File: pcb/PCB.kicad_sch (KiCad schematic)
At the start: 35 parts, among them J1 Conn_01x15, J2 USB_C_Receptacle_USB2.0, J3 Conn_01x15, J4 TC2030, J5 Conn_01x04, SW1 SW_Push, SW2 SW_Push, U1 SN65HVD230, U2 AMS1117-3.3, U3 STM32F103C8T6, Y1 8MHz

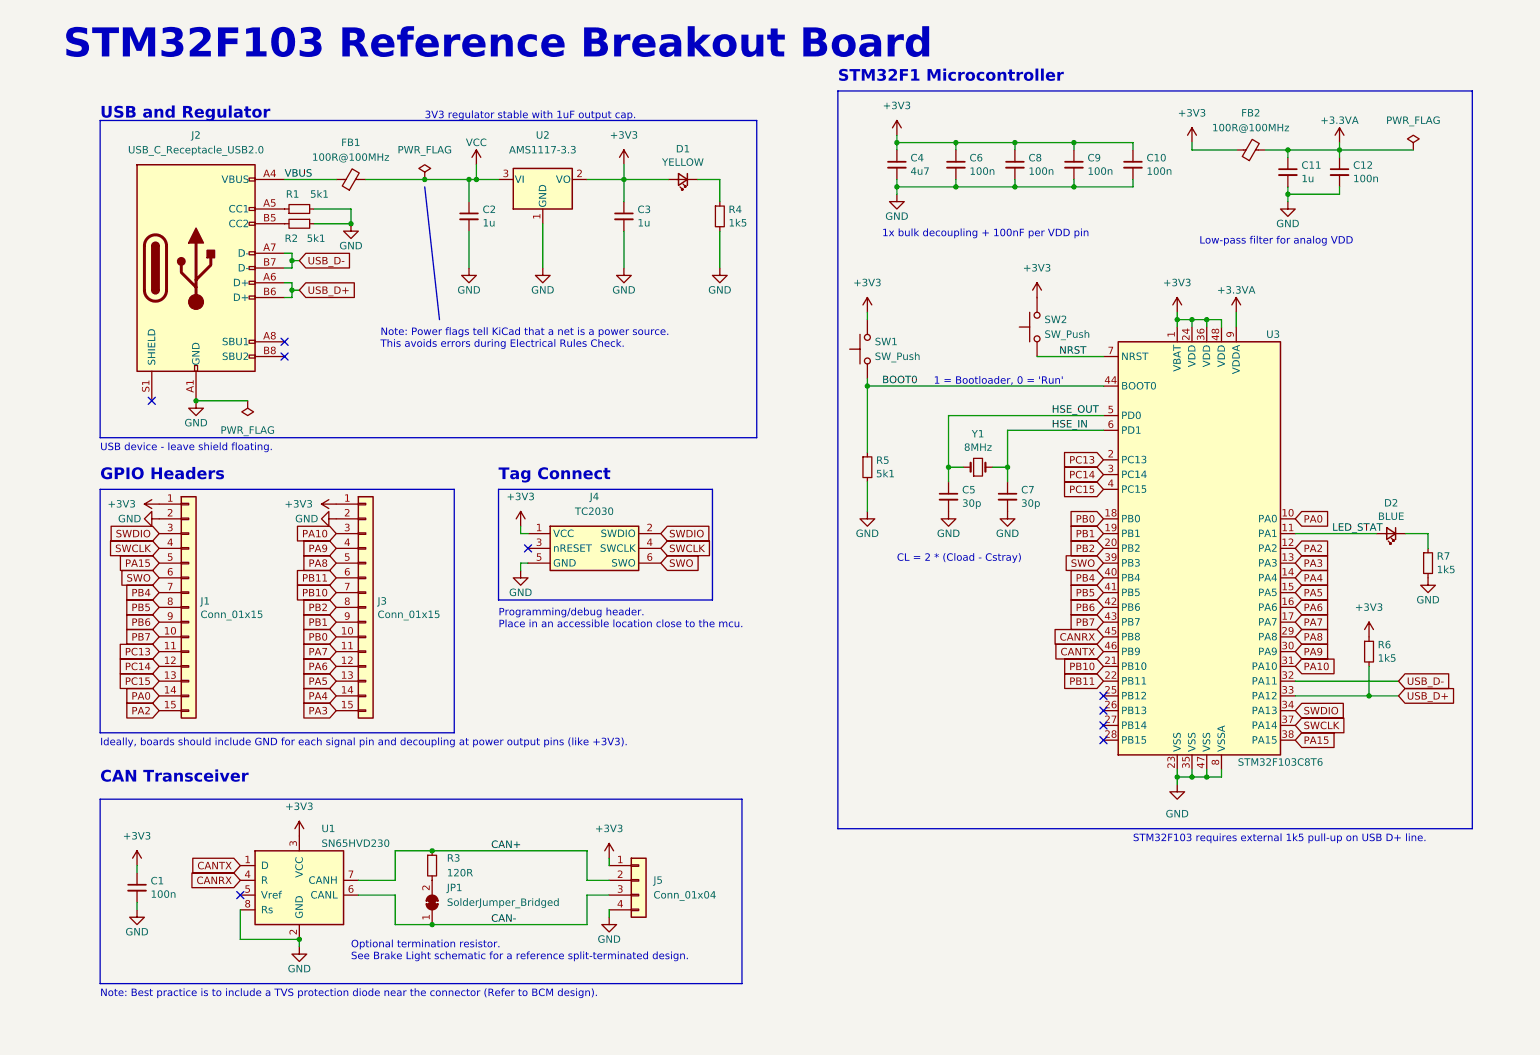
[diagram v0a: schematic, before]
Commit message: Finished schematic
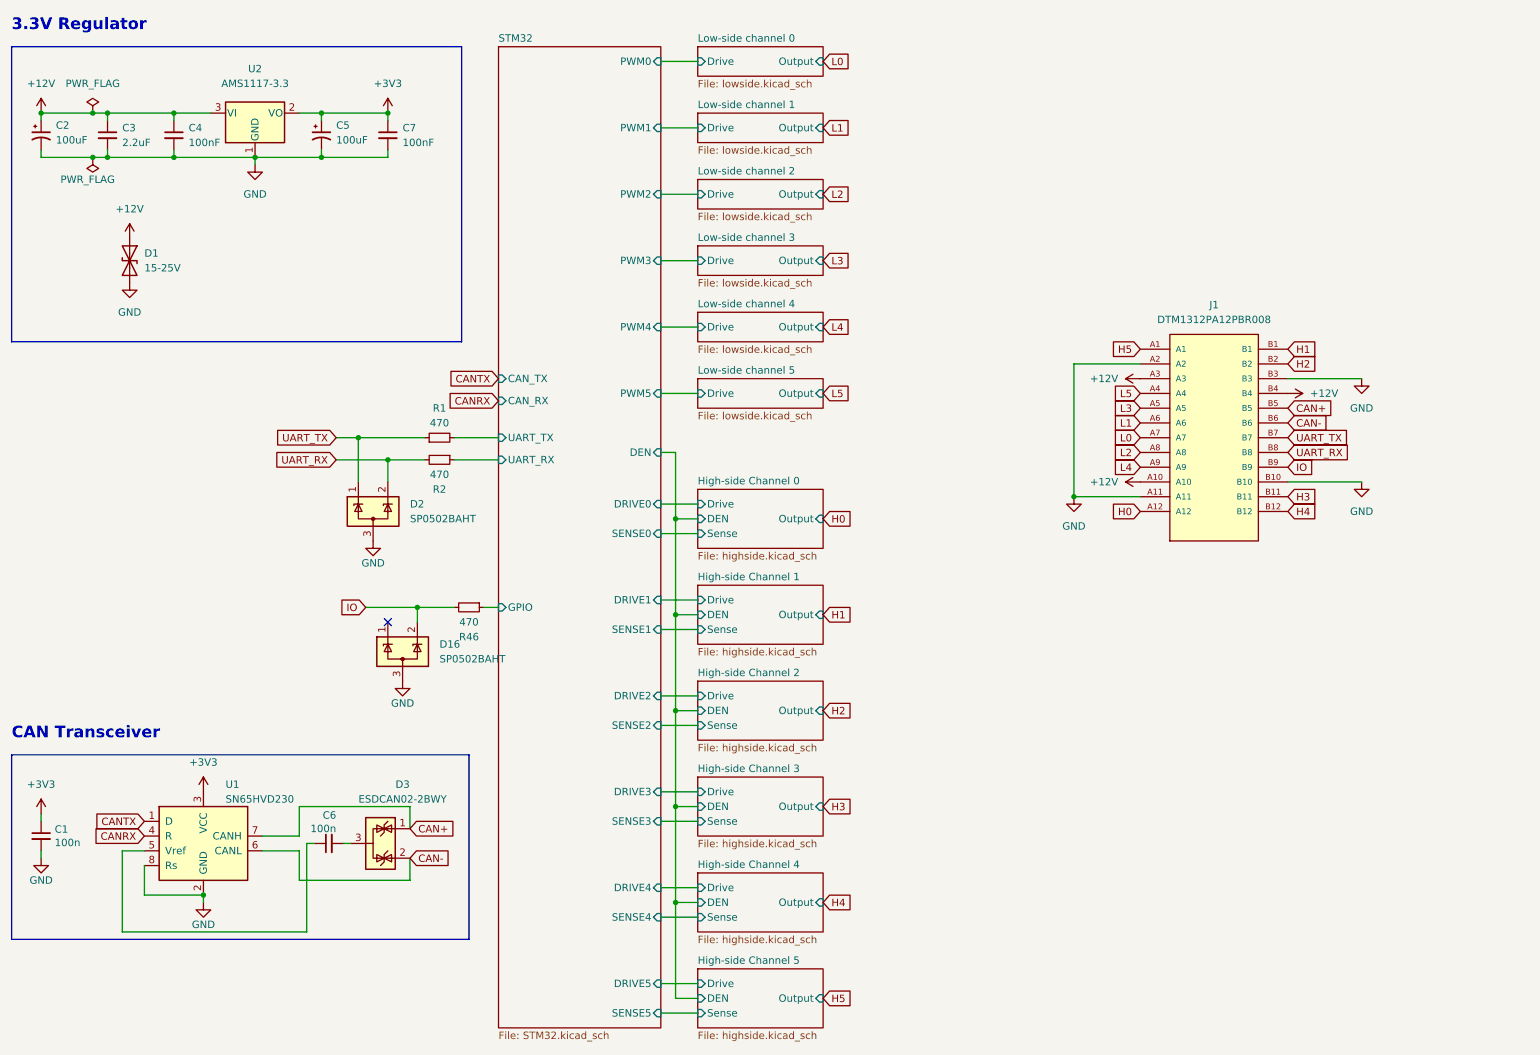
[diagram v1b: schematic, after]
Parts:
- removed C10, C12, C8, C9: 100n, Capacitor_SMD:C_0402_1005Metric, symbol Device:C_Small
- removed C11, C2: 1u, Capacitor_SMD:C_0603_1608Metric, symbol Device:C_Small
- removed C5: 30p, Capacitor_SMD:C_0402_1005Metric, symbol Device:C_Small
- removed D1: YELLOW, LED_SMD:LED_0603_1608Metric, symbol Device:LED_Small
- removed D2: BLUE, LED_SMD:LED_0603_1608Metric, symbol Device:LED_Small
- removed FB1, FB2: 100R@100MHz, Resistor_SMD:R_0805_2012Metric, symbol Device:FerriteBead_Small
- removed J1, J3: Conn_01x15, Connector_PinHeader_2.54mm:PinHeader_1x15_P2.54mm_Vertical, symbol Connector_Generic:Conn_01x15
- removed J2: USB_C_Receptacle_USB2.0, Connector_USB:USB_C_Receptacle_HRO_TYPE-C-31-M-12, symbol Connector:USB_C_Receptacle_USB2.0
- removed J4: TC2030, Connector:Tag-Connect_TC2030-IDC-NL_2x03_P1.27mm_Vertical, symbol TC2030:TC2030
- removed J5: Conn_01x04, Connector_PinHeader_2.54mm:PinHeader_1x04_P2.54mm_Vertical, symbol Connector_Generic:Conn_01x04
- removed JP1: SolderJumper_Bridged, Jumper:SolderJumper-2_P1.3mm_Bridged_RoundedPad1.0x1.5mm, symbol Jumper:SolderJumper_2_Bridged
- removed R3: 120R, Resistor_SMD:R_0402_1005Metric, symbol Device:R_Small
- removed R4, R6, R7: 1k5, Resistor_SMD:R_0402_1005Metric, symbol Device:R_Small
- removed R5: 5k1, Resistor_SMD:R_0402_1005Metric, symbol Device:R_Small
- removed SW1, SW2: SW_Push, Button_Switch_SMD:SW_Push_1P1T_NO_CK_KSC7xxJ, symbol Switch:SW_Push
- removed U3: STM32F103C8T6, Package_QFP:LQFP-48_7x7mm_P0.5mm, symbol MCU_ST_STM32F1:STM32F103C8Tx
- removed Y1: 8MHz, Crystal:Crystal_SMD_5032-2Pin_5.0x3.2mm, symbol Device:Crystal_Small
- added C2, C5: 100uF, Capacitor_SMD:CP_Elec_6.3x7.7, symbol Device:C_Polarized_Small_US
- added D1: 15-25V, Diode_SMD:D_SMA, symbol Device:D_TVS
- added D16, D2: SP0502BAHT, Package_TO_SOT_SMD:SOT-23, symbol Power_Protection:SP0502BAHT
- added D3: ESDCAN02-2BWY, Package_TO_SOT_SMD:SOT-23, symbol Power_Protection:NUP2105L
- added J1: DTM1312PA12PBR008, DTM13-12PA-12PB:TE_DTM1312PA12PBR008, symbol DTM1312PA12PBR008:DTM1312PA12PBR008
- added R46: 470, Resistor_SMD:R_0603_1608Metric, symbol Device:R_Small
- C3: value 1u -> 2.2uF; footprint Capacitor_SMD:C_0603_1608Metric -> Capacitor_SMD:C_0805_2012Metric; LCSC C15849 -> (none)
- C4: value 4u7 -> 100nF; LCSC C19666 -> (none)
- C7: value 30p -> 100nF; footprint Capacitor_SMD:C_0402_1005Metric -> Capacitor_SMD:C_0603_1608Metric; LCSC C1570 -> (none)
- R1, R2: value 5k1 -> 470; footprint Resistor_SMD:R_0402_1005Metric -> Resistor_SMD:R_0603_1608Metric; LCSC C25905 -> (none)
- U2: LCSC C6186 -> (none)
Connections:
- net HSE_IN is gone; now on net +3V3: C7.1
- net +3V3: now also C5.1; no longer C3.1, C4.1, C6.1
- net CAN+: now also D3.1 (K), J1.B5
- net CAN-: now also D3.2 (K), J1.B6
- net GND: now also C2.2, C5.2, D1.2 (A2), D16.3 (A), D2.3 (A), J1.A11, J1.A2, J1.B10, J1.B3; no longer C6.2, R1.2, R2.1
- net UART_TX: now reaches R1.1
- net UART_TX: now also D2.1 (K), J1.B7
- net UART_RX: now reaches R2.2
- net UART_RX: now also D2.2 (K), J1.B8
- net at U1.5 (Vref): now also C6.1
- net VCC renamed +12V
- net +12V: now also C3.1, C4.1, C2.1, D1.1 (A1), J1.A10, J1.A3, J1.B4
- new net: C6.2, D3.3 (A)
- new net H0: J1.A12
- new net H1: J1.B1
- new net H2: J1.B2
- new net H3: J1.B11
- new net H4: J1.B12
- new net H5: J1.A1
- new net IO: D16.2 (K), J1.B9, R46.2
- new net L0: J1.A7
- new net L1: J1.A6
- new net L2: J1.A8
- new net L3: J1.A5
- new net L4: J1.A9
- new net L5: J1.A4
- new net STM32/GPIO: R46.1
- new net STM32/UART_RX: R2.1
- new net STM32/UART_TX: R1.2
- no-connect marks 9 -> 1
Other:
- added sheet High-side Channel 0 (highside.kicad_sch)
- added sheet High-side Channel 1 (highside.kicad_sch)
- added sheet High-side Channel 2 (highside.kicad_sch)
- added sheet High-side Channel 3 (highside.kicad_sch)
- added sheet High-side Channel 4 (highside.kicad_sch)
- added sheet High-side Channel 5 (highside.kicad_sch)
- added sheet Low-side channel 0 (lowside.kicad_sch)
- added sheet Low-side channel 1 (lowside.kicad_sch)
- added sheet Low-side channel 2 (lowside.kicad_sch)
- added sheet Low-side channel 3 (lowside.kicad_sch)
- added sheet Low-side channel 4 (lowside.kicad_sch)
- added sheet Low-side channel 5 (lowside.kicad_sch)
- added sheet STM32 (STM32.kicad_sch)
- note added: "3.3V Regulator"
- note removed: "1 = Bootloader, 0 = 'Run'"
- note removed: "1x bulk decoupling + 100nF per VDD pin"
- note removed: "3V3 regulator stable with 1uF output cap."
- note removed: "CL = 2 * (Cload - Cstray)"
- note removed: "GPIO Headers"
- note removed: "Ideally, boards should include GND for each signal pin and decoupling at power output pins (like +3V3)."
- note removed: "Low-pass filter for analog VDD"
- note removed: "Note: Best practice is to include a TVS protection diode near the connector (Refer to BCM design)."
- note removed: "Note: Power flags tell KiCad that a net is a power source. This avoids errors during Electrical Rules Check."
- note removed: "Optional termination resistor. See Brake Light schematic for a reference split-terminated design."
- note removed: "Programming/debug header. Place in an accessible location close to the mcu."
- note removed: "STM32F1 Microcontroller"
- note removed: "STM32F103 Reference Breakout Board"
- note removed: "STM32F103 requires external 1k5 pull-up on USB D+ line."
- note removed: "Tag Connect"
- note removed: "USB and Regulator"
- note removed: "USB device - leave shield floating."
- moved on the sheet: C1, U1
